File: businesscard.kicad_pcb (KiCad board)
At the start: 2 copper layers, 88.9 x 50.8 mm, 6 parts

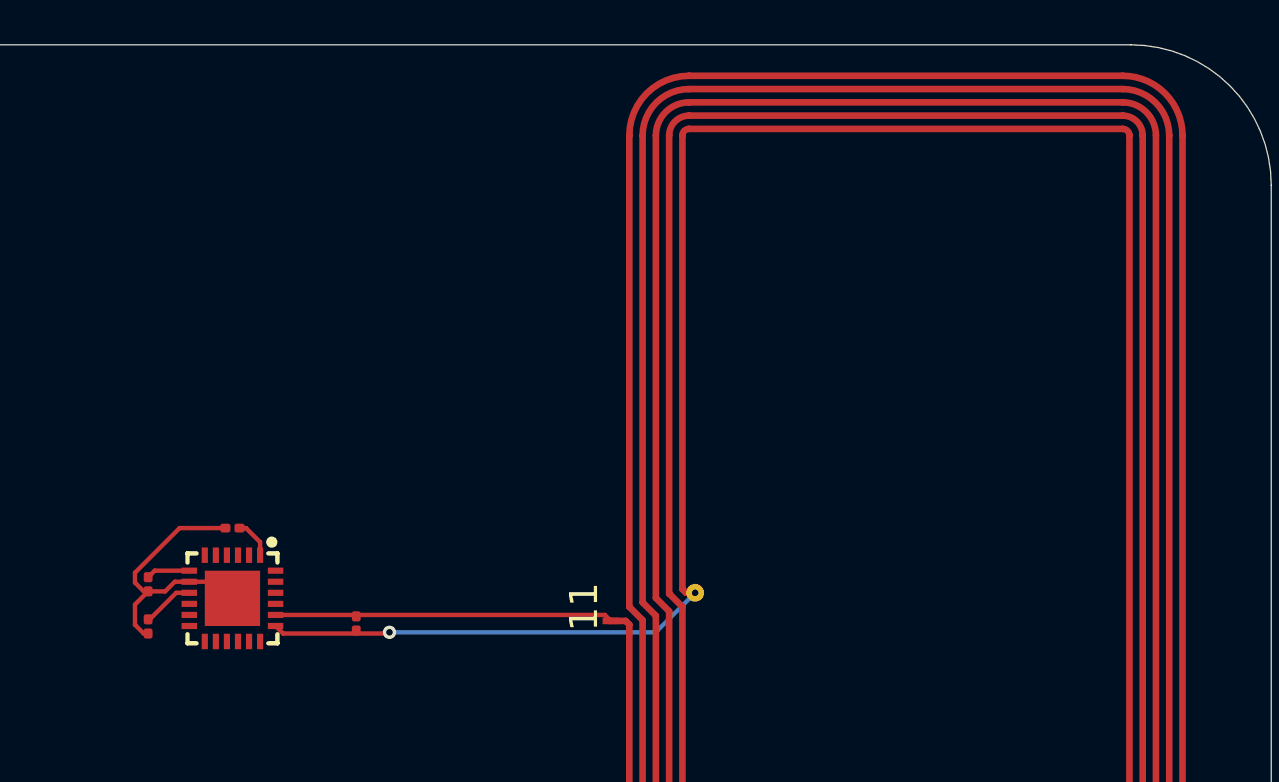
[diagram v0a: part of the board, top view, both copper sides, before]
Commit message: stuff
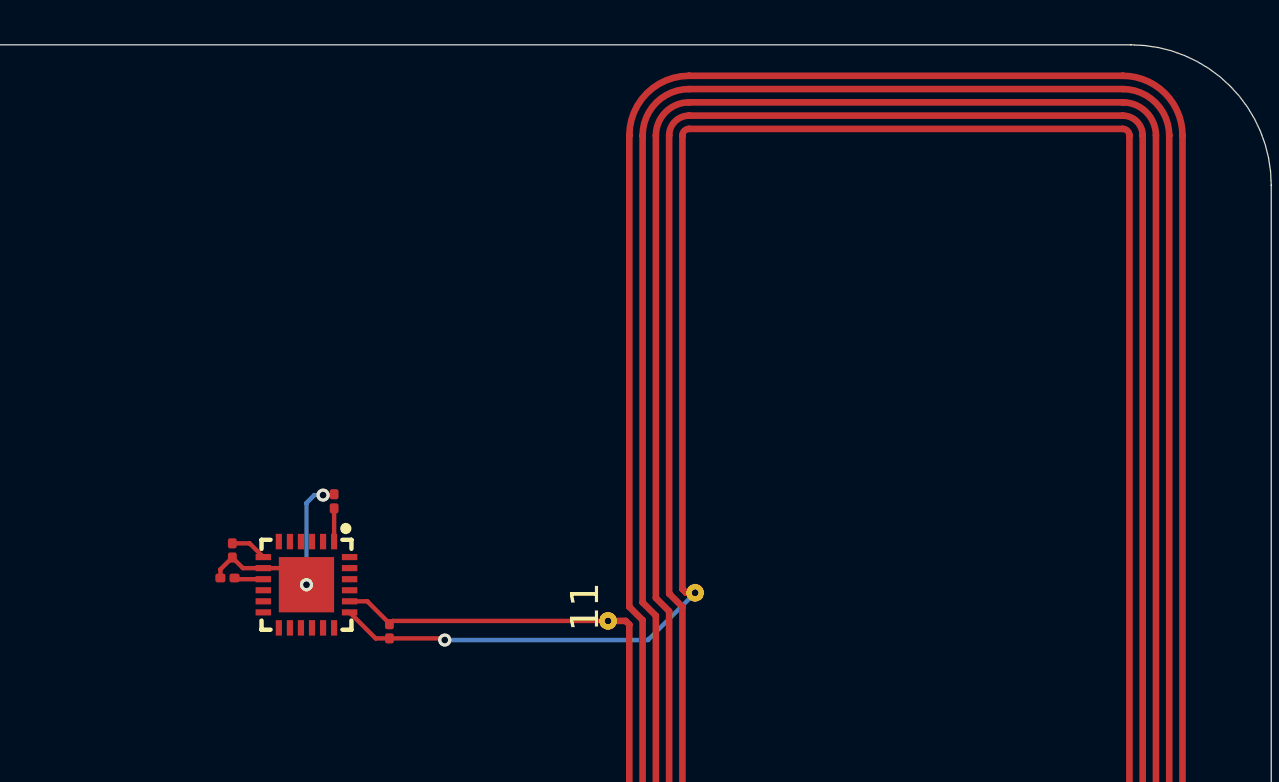
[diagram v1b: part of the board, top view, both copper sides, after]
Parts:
- moved C4 4.75 mm to (154.5, 90.5), turned to 90 degrees
- moved C3 4.20 mm to (149.7, 93.9), turned to 180 degrees
- moved C2 4.10 mm to (149.9, 92.7)
- moved U2 3.40 mm to (153.2, 94.2)
- moved C1 1.54 mm to (157.0, 96.4)
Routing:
- net Net-(U2-LA): track 15.3 -> 12.2 mm
- net Net-(U2-LB): track 19.9 -> 17.0 mm
- net GND: track 12.9 -> 10.1 mm, vias 0 -> 2
- net Net-(U2-RESETN): track 2.36 -> 1.32 mm
